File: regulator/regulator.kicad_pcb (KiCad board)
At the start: 2 copper layers, 53.3 x 27.9 mm, 23 parts, among them J1 02x03, J1 03x03, J1 04x07, J1 Conn_01x02, J2 Conn_01x02, J4 Barrel_Jack_Switch, J5 Barrel_Jack_Switch, J6 Conn_01x02, J7 Conn_01x02, J8 Conn_01x02

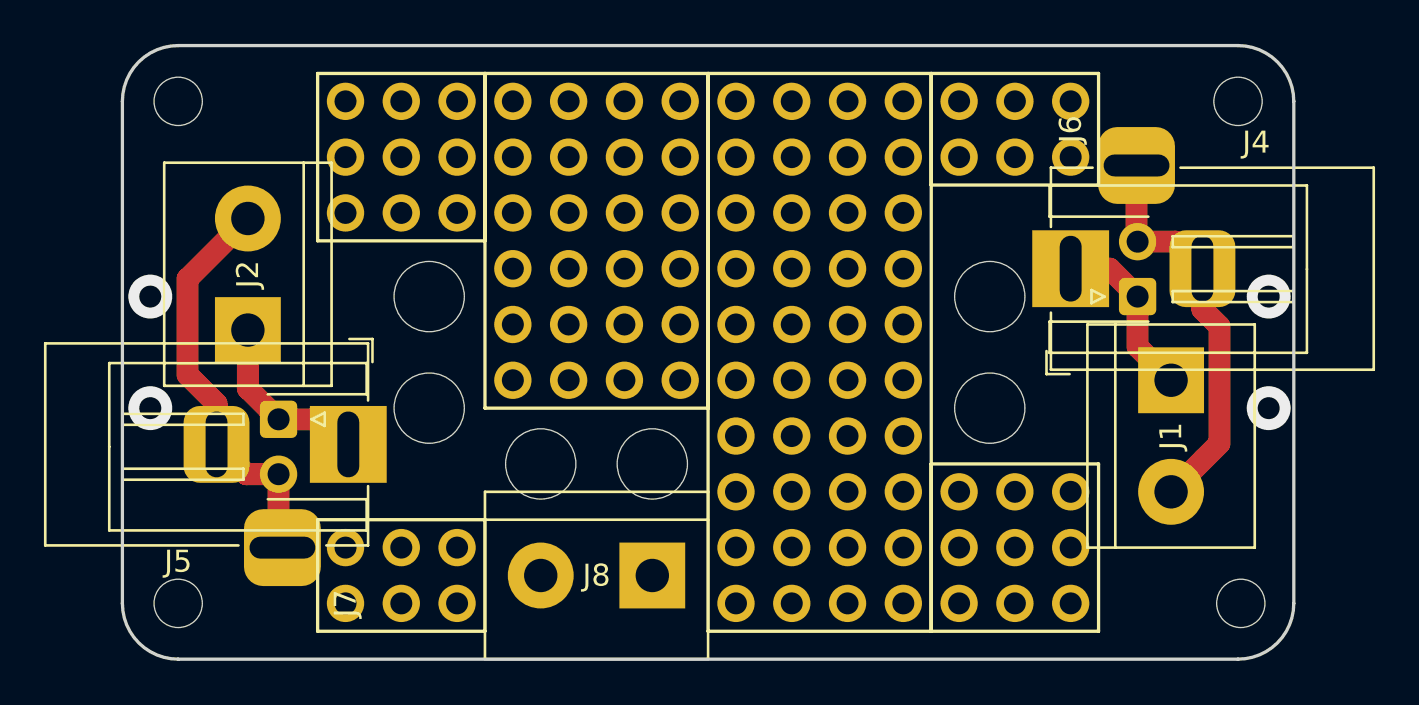
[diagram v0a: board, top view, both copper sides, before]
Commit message: regulator update
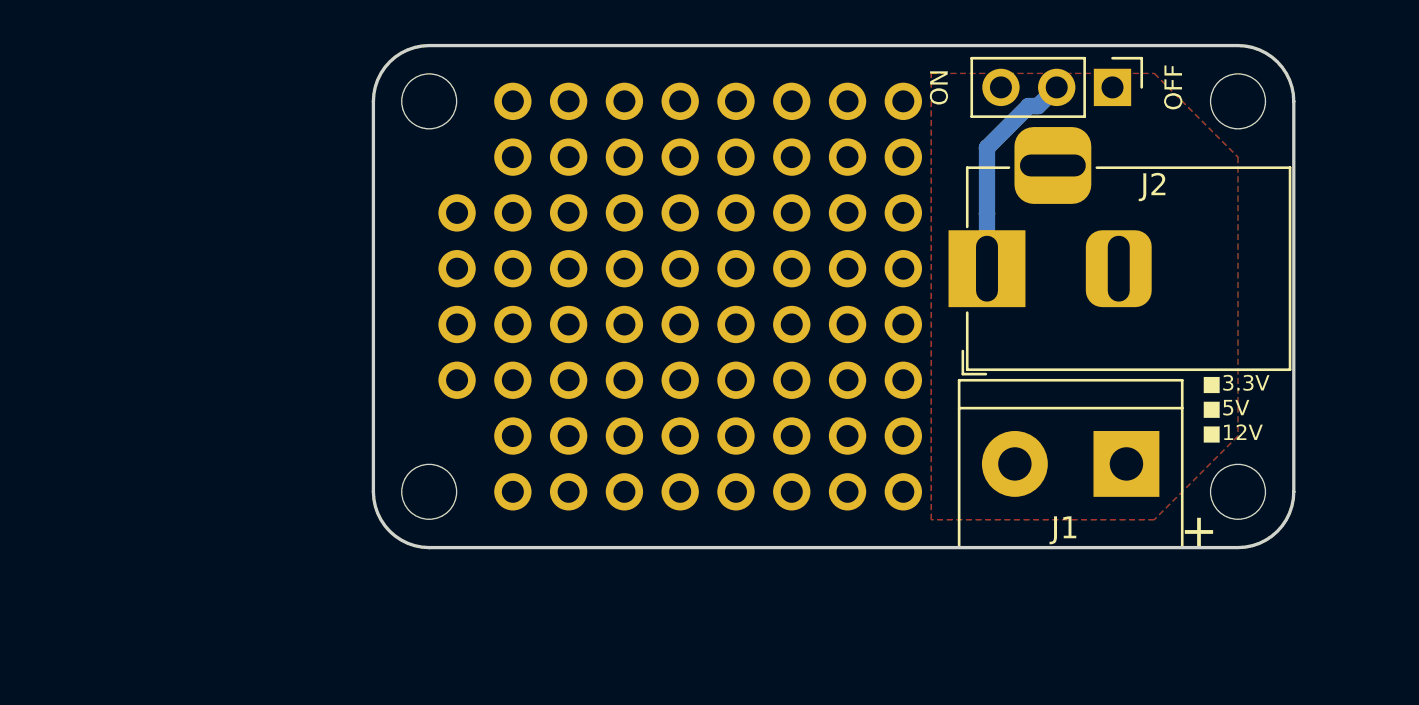
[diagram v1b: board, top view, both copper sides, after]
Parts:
- removed the J1 at (179.1, 88.9)
- removed the J1 at (166.4, 88.9)
- removed the J1 at (176.5, 88.9)
- removed the J1 at (188.7, 101.6)
- removed the J1 at (184.2, 106.7)
- removed the J1 at (156.2, 88.9)
- removed the J1 at (151.1, 109.2)
- removed J4, J5: Barrel_Jack_Switch, Connector_BarrelJack:BarrelJack_Horizontal
- removed J6, J7: Conn_01x02, Connector_JST:JST_XH_S02B-XH-A-1_1x02_P2.50mm_Horizontal
- removed J8: Conn_01x02, TerminalBlock:TerminalBlock_bornier-2_P5.08mm
- removed the REF** at (160.0, 105.4)
- removed the REF** at (154.9, 97.8)
- removed the REF** at (165.1, 105.4)
- removed the REF** at (180.5, 102.9)
- removed the REF** at (180.5, 97.8)
- removed the REF** at (154.9, 102.9)
- removed the REF** at (191.8, 88.9)
- removed the REF** at (191.9, 111.8)
- removed the REF** at (143.5, 88.9)
- removed the REF** at (143.5, 111.8)
- added J1: Conn_01x02, TerminalBlock:TerminalBlock_bornier-2_P5.08mm, F.Cu at (186.7, 105.4)
- added J1: 0x04, lib:Prototype_Area_2.54mm_01x04, F.Cu at (156.2, 94.0)
- added J10: 09x10, lib:Prototype_Area_2.54mm_08x08, F.Cu at (176.5, 88.9)
- added REF**: MountingHole_2.5mm, MountingHole:MountingHole_2.5mm, F.Cu at (154.9, 106.7)
- added REF**: MountingHole_2.5mm, MountingHole:MountingHole_2.5mm, F.Cu at (154.9, 88.9)
- added REF**: MountingHole_2.5mm, MountingHole:MountingHole_2.5mm, F.Cu at (191.8, 106.7)
- added REF**: MountingHole_2.5mm, MountingHole:MountingHole_2.5mm, F.Cu at (191.8, 88.9)
- added SW1: SW_SPDT, Connector_PinHeader_2.54mm:PinHeader_1x03_P2.54mm_Vertical, F.Cu at (186.1, 88.3)
- J2: value Conn_01x02 -> Barrel_Jack_Switch; footprint TerminalBlock:TerminalBlock_bornier-2_P5.08mm -> Connector_BarrelJack:BarrelJack_Horizontal
- moved J2 33.8 mm to (180.3, 96.5), turned to 180 degrees
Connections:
- J2 pad 2: Net-(J2-Pad2) -> GND
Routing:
- net Net-(J2-Pad2): track 18.8 -> 0.00 mm
- net Net-(J1-Pad2): track 18.3 -> 0.00 mm
- net Net-(J1-Pad1): track 8.02 -> 0.00 mm
- net Net-(J2-Pad1): track 8.29 -> 9.82 mm
- net (no net): vias 4 -> 0
- added copper zone on F.Cu, net GND
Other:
- board size 53.3 x 27.9 mm -> 41.9 x 22.9 mm
- net class Default: trace_width 1 -> 0.75
- board text added: "+"
- board text added: "OFF"
- board text added: "ON"
- board text added: "■3.3V ■5V ■12V"
